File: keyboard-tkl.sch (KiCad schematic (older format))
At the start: 108 parts, among them P1 USB_OTG, P2 JTAG, U1 AT32UC3B1512, U2 74HC595, U3 74HC595, U4 74HC595, U5 LD1117S33CTR, Y1 12MHz

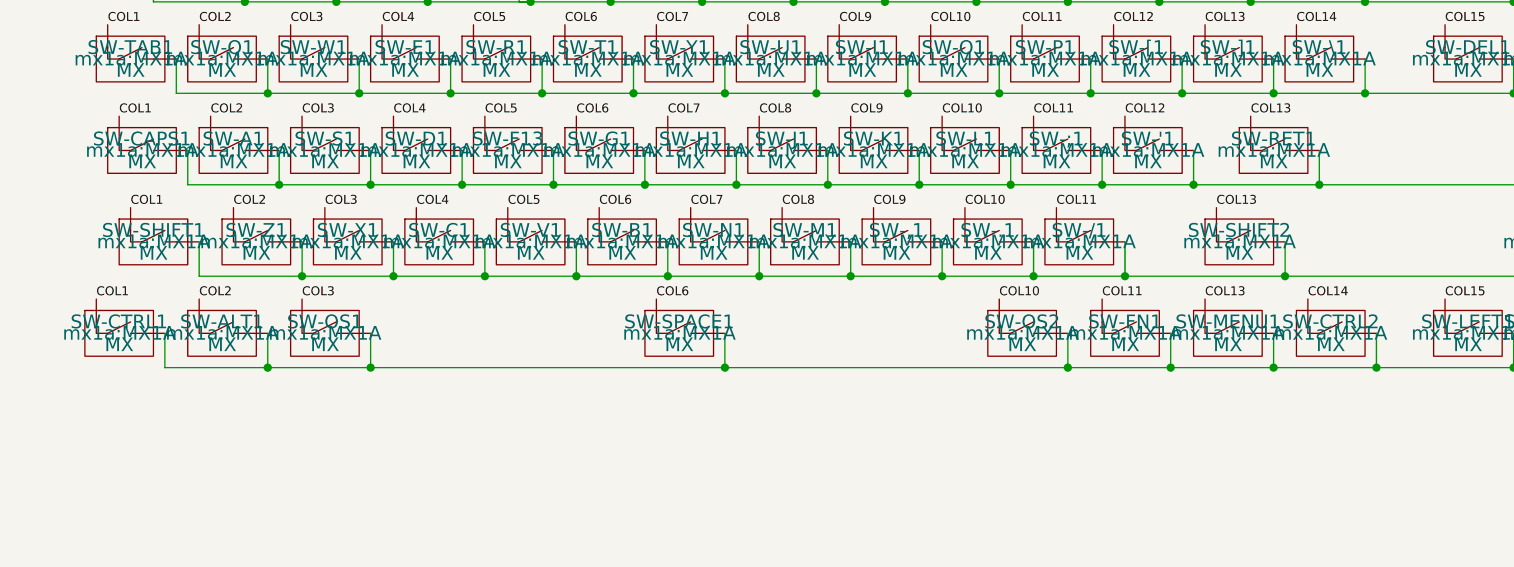
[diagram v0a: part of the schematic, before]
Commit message: Add stabs to big keys
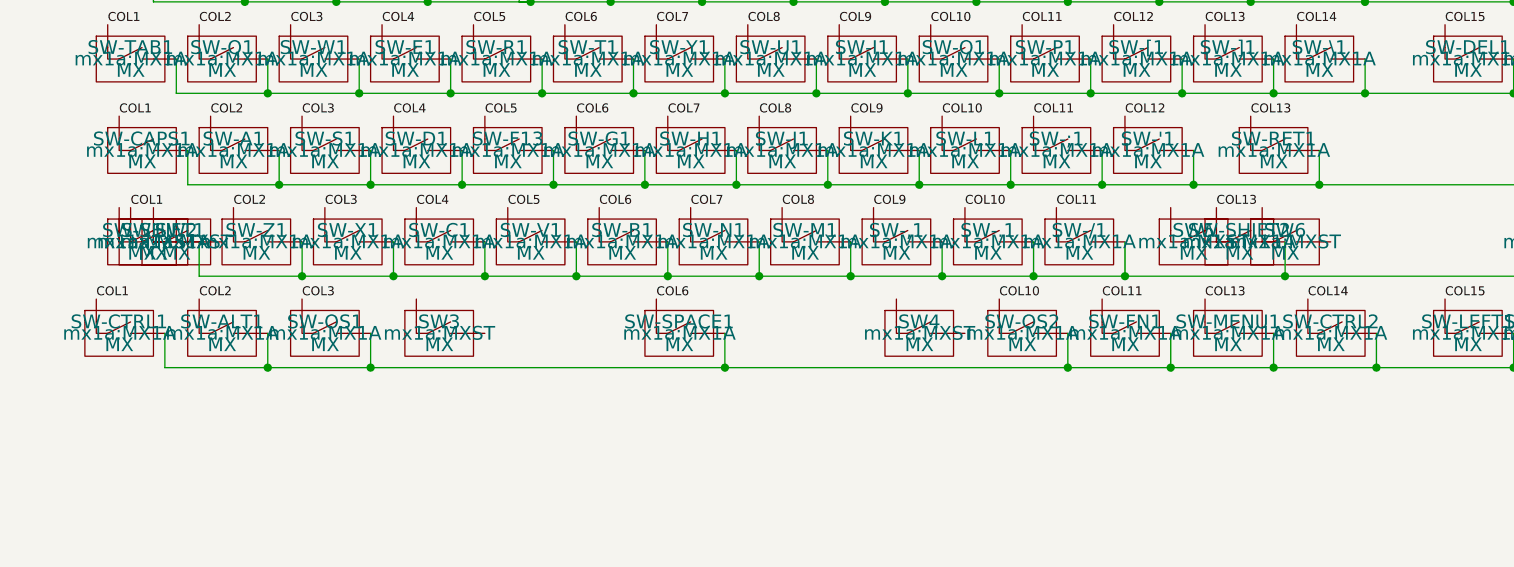
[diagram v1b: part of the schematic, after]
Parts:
- added SW1, SW2, SW3, SW4, SW5, SW6: MX, mx1a:MXST, symbol MX
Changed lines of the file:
@@
 Wire Wire Line
 	10750 950  10750 1150
+$Comp
+L MX SW3
+U 1 1 55E28F84
+P 2450 2900
+F 0 "SW3" H 2450 2950 60  0000 C CNN
+F 1 "MX" H 2450 2850 60  0000 C CNN
+F 2 "mx1a:MXST" H 2450 2900 60  0000 C CNN
+F 3 "" H 2450 2900 60  0000 C CNN
+	1    2450 2900
+	1    0    0    -1
+$EndComp
+$Comp
+L MX SW4
+U 1 1 55E296F8
+P 4550 2900
+F 0 "SW4" H 4550 2950 60  0000 C CNN
+F 1 "MX" H 4550 2850 60  0000 C CNN
+F 2 "mx1a:MXST" H 4550 2900 60  0000 C CNN
+F 3 "" H 4550 2900 60  0000 C CNN
+	1    4550 2900
+	1    0    0    -1
+$EndComp
+$Comp
+L MX SW6
+U 1 1 55E29E84
+P 6150 2500
+F 0 "SW6" H 6150 2550 60  0000 C CNN
+F 1 "MX" H 6150 2450 60  0000 C CNN
+F 2 "mx1a:MXST" H 6150 2500 60  0000 C CNN
+F 3 "" H 6150 2500 60  0000 C CNN
+	1    6150 2500
+	1    0    0    -1
+$EndComp
+$Comp
+L MX SW5
+U 1 1 55E2A005
+P 5750 2500
+F 0 "SW5" H 5750 2550 60  0000 C CNN
+F 1 "MX" H 5750 2450 60  0000 C CNN
+F 2 "mx1a:MXST" H 5750 2500 60  0000 C CNN
+F 3 "" H 5750 2500 60  0000 C CNN
+	1    5750 2500
+	1    0    0    -1
+$EndComp
+$Comp
+L MX SW1
+U 1 1 55E2A3B8
+P 1150 2500
+F 0 "SW1" H 1150 2550 60  0000 C CNN
+F 1 "MX" H 1150 2450 60  0000 C CNN
+F 2 "mx1a:MXST" H 1150 2500 60  0000 C CNN
+F 3 "" H 1150 2500 60  0000 C CNN
+	1    1150 2500
+	1    0    0    -1
+$EndComp
+$Comp
+L MX SW2
+U 1 1 55E2A529
+P 1300 2500
+F 0 "SW2" H 1300 2550 60  0000 C CNN
+F 1 "MX" H 1300 2450 60  0000 C CNN
+F 2 "mx1a:MXST" H 1300 2500 60  0000 C CNN
+F 3 "" H 1300 2500 60  0000 C CNN
+	1    1300 2500
+	1    0    0    -1
+$EndComp
 $EndSCHEMATC
